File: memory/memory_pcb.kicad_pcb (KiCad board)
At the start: 2 copper layers, 116.8 x 56.6 mm, 43 parts, among them J1 Conn_02x01, J2 Conn_02x02_Odd_Even, J3 Conn_02x08_Odd_Even, J4 Conn_02x08_Odd_Even, U1 74LS04, U2 AT28C256-15PU, U3 AT28C256-15PU, U4 74LS245, U5 74LS245

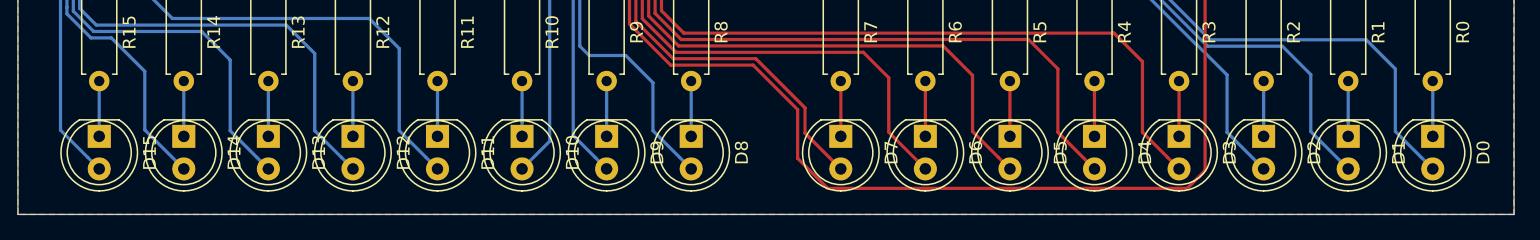
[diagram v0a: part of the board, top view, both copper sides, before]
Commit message: program counter
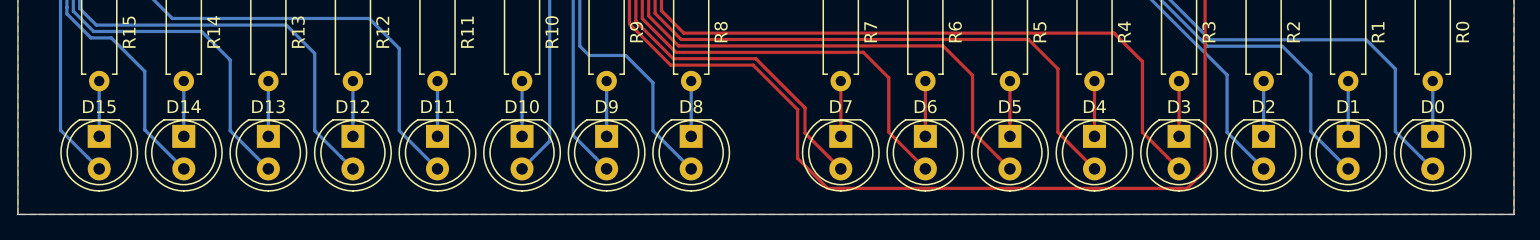
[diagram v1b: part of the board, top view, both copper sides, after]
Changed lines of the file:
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@@
     (descr "LED, diameter 5.0mm, 2 pins, http://cdn-reichelt.de/documents/datenblatt/A500/LL-504BC2E-009.pdf")
     (tags "LED diameter 5.0mm 2 pins")
-    (fp_text reference D0 (at 1.27 -3.96 90) (layer F.SilkS)
+    (fp_text reference D0 (at -2.286 0 180) (layer F.SilkS)
       (effects (font (size 1 1) (thickness 0.15)))
     )
@@
     (descr "LED, diameter 5.0mm, 2 pins, http://cdn-reichelt.de/documents/datenblatt/A500/LL-504BC2E-009.pdf")
     (tags "LED diameter 5.0mm 2 pins")
-    (fp_text reference D1 (at 1.27 -3.96 90) (layer F.SilkS)
+    (fp_text reference D1 (at -2.286 0 180) (layer F.SilkS)
       (effects (font (size 1 1) (thickness 0.15)))
     )
@@
     (descr "LED, diameter 5.0mm, 2 pins, http://cdn-reichelt.de/documents/datenblatt/A500/LL-504BC2E-009.pdf")
     (tags "LED diameter 5.0mm 2 pins")
-    (fp_text reference D2 (at 1.27 -3.96 90) (layer F.SilkS)
+    (fp_text reference D2 (at -2.286 0 180) (layer F.SilkS)
       (effects (font (size 1 1) (thickness 0.15)))
     )
@@
     (descr "LED, diameter 5.0mm, 2 pins, http://cdn-reichelt.de/documents/datenblatt/A500/LL-504BC2E-009.pdf")
     (tags "LED diameter 5.0mm 2 pins")
-    (fp_text reference D3 (at 1.27 -3.96 90) (layer F.SilkS)
+    (fp_text reference D3 (at -2.286 0 180) (layer F.SilkS)
       (effects (font (size 1 1) (thickness 0.15)))
     )
@@
     (descr "LED, diameter 5.0mm, 2 pins, http://cdn-reichelt.de/documents/datenblatt/A500/LL-504BC2E-009.pdf")
     (tags "LED diameter 5.0mm 2 pins")
-    (fp_text reference D4 (at 1.27 -3.96 90) (layer F.SilkS)
+    (fp_text reference D4 (at -2.286 0 180) (layer F.SilkS)
       (effects (font (size 1 1) (thickness 0.15)))
     )
@@
     (descr "LED, diameter 5.0mm, 2 pins, http://cdn-reichelt.de/documents/datenblatt/A500/LL-504BC2E-009.pdf")
     (tags "LED diameter 5.0mm 2 pins")
-    (fp_text reference D5 (at 1.27 -3.96 90) (layer F.SilkS)
+    (fp_text reference D5 (at -2.286 0 180) (layer F.SilkS)
       (effects (font (size 1 1) (thickness 0.15)))
     )
@@
     (descr "LED, diameter 5.0mm, 2 pins, http://cdn-reichelt.de/documents/datenblatt/A500/LL-504BC2E-009.pdf")
     (tags "LED diameter 5.0mm 2 pins")
-    (fp_text reference D6 (at 1.27 -3.96 90) (layer F.SilkS)
+    (fp_text reference D6 (at -2.286 0 180) (layer F.SilkS)
       (effects (font (size 1 1) (thickness 0.15)))
     )
@@
     (descr "LED, diameter 5.0mm, 2 pins, http://cdn-reichelt.de/documents/datenblatt/A500/LL-504BC2E-009.pdf")
     (tags "LED diameter 5.0mm 2 pins")
-    (fp_text reference D7 (at 1.27 -3.96 90) (layer F.SilkS)
+    (fp_text reference D7 (at -2.286 0 180) (layer F.SilkS)
       (effects (font (size 1 1) (thickness 0.15)))
     )
@@
     (descr "LED, diameter 5.0mm, 2 pins, http://cdn-reichelt.de/documents/datenblatt/A500/LL-504BC2E-009.pdf")
     (tags "LED diameter 5.0mm 2 pins")
-    (fp_text reference D8 (at 1.27 -3.96 90) (layer F.SilkS)
+    (fp_text reference D8 (at -2.286 0 180) (layer F.SilkS)
       (effects (font (size 1 1) (thickness 0.15)))
     )
@@
     (descr "LED, diameter 5.0mm, 2 pins, http://cdn-reichelt.de/documents/datenblatt/A500/LL-504BC2E-009.pdf")
     (tags "LED diameter 5.0mm 2 pins")
-    (fp_text reference D9 (at 1.27 -3.96 90) (layer F.SilkS)
+    (fp_text reference D9 (at -2.286 0 180) (layer F.SilkS)
       (effects (font (size 1 1) (thickness 0.15)))
     )
@@
     (descr "LED, diameter 5.0mm, 2 pins, http://cdn-reichelt.de/documents/datenblatt/A500/LL-504BC2E-009.pdf")
     (tags "LED diameter 5.0mm 2 pins")
-    (fp_text reference D10 (at 1.27 -3.96 90) (layer F.SilkS)
+    (fp_text reference D10 (at -2.286 0 180) (layer F.SilkS)
       (effects (font (size 1 1) (thickness 0.15)))
     )
@@
     (descr "LED, diameter 5.0mm, 2 pins, http://cdn-reichelt.de/documents/datenblatt/A500/LL-504BC2E-009.pdf")
     (tags "LED diameter 5.0mm 2 pins")
-    (fp_text reference D11 (at 1.27 -3.96 90) (layer F.SilkS)
+    (fp_text reference D11 (at -2.286 0 180) (layer F.SilkS)
       (effects (font (size 1 1) (thickness 0.15)))
     )
@@
     (descr "LED, diameter 5.0mm, 2 pins, http://cdn-reichelt.de/documents/datenblatt/A500/LL-504BC2E-009.pdf")
     (tags "LED diameter 5.0mm 2 pins")
-    (fp_text reference D12 (at 1.27 -3.96 90) (layer F.SilkS)
+    (fp_text reference D12 (at -2.286 0 180) (layer F.SilkS)
       (effects (font (size 1 1) (thickness 0.15)))
     )
@@
     (descr "LED, diameter 5.0mm, 2 pins, http://cdn-reichelt.de/documents/datenblatt/A500/LL-504BC2E-009.pdf")
     (tags "LED diameter 5.0mm 2 pins")
-    (fp_text reference D13 (at 1.27 -3.96 90) (layer F.SilkS)
+    (fp_text reference D13 (at -2.286 0 180) (layer F.SilkS)
       (effects (font (size 1 1) (thickness 0.15)))
     )
@@
     (descr "LED, diameter 5.0mm, 2 pins, http://cdn-reichelt.de/documents/datenblatt/A500/LL-504BC2E-009.pdf")
     (tags "LED diameter 5.0mm 2 pins")
-    (fp_text reference D14 (at 1.27 -3.96 90) (layer F.SilkS)
+    (fp_text reference D14 (at -2.286 0 180) (layer F.SilkS)
       (effects (font (size 1 1) (thickness 0.15)))
     )
@@
     (descr "LED, diameter 5.0mm, 2 pins, http://cdn-reichelt.de/documents/datenblatt/A500/LL-504BC2E-009.pdf")
     (tags "LED diameter 5.0mm 2 pins")
-    (fp_text reference D15 (at 1.27 -3.96 90) (layer F.SilkS)
-      (effects (font (size 1 1) (thickness 0.15)))
-    )
+    (fp_text reference D15 (at -2.286 0 180) (layer F.SilkS)
+      (effects (font (size 1 1) (thickness 0.15)))
+    )
